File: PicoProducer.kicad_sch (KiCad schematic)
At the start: 37 parts, among them SW1 cherry_mx, SW10 cherry_mx, SW11 cherry_mx, SW12 cherry_mx, SW2 cherry_mx, SW3 cherry_mx, SW4 cherry_mx, SW5 cherry_mx, SW6 cherry_mx, SW7 cherry_mx, SW8 cherry_mx, SW9 cherry_mx, U1 RPI_PICO-SMD

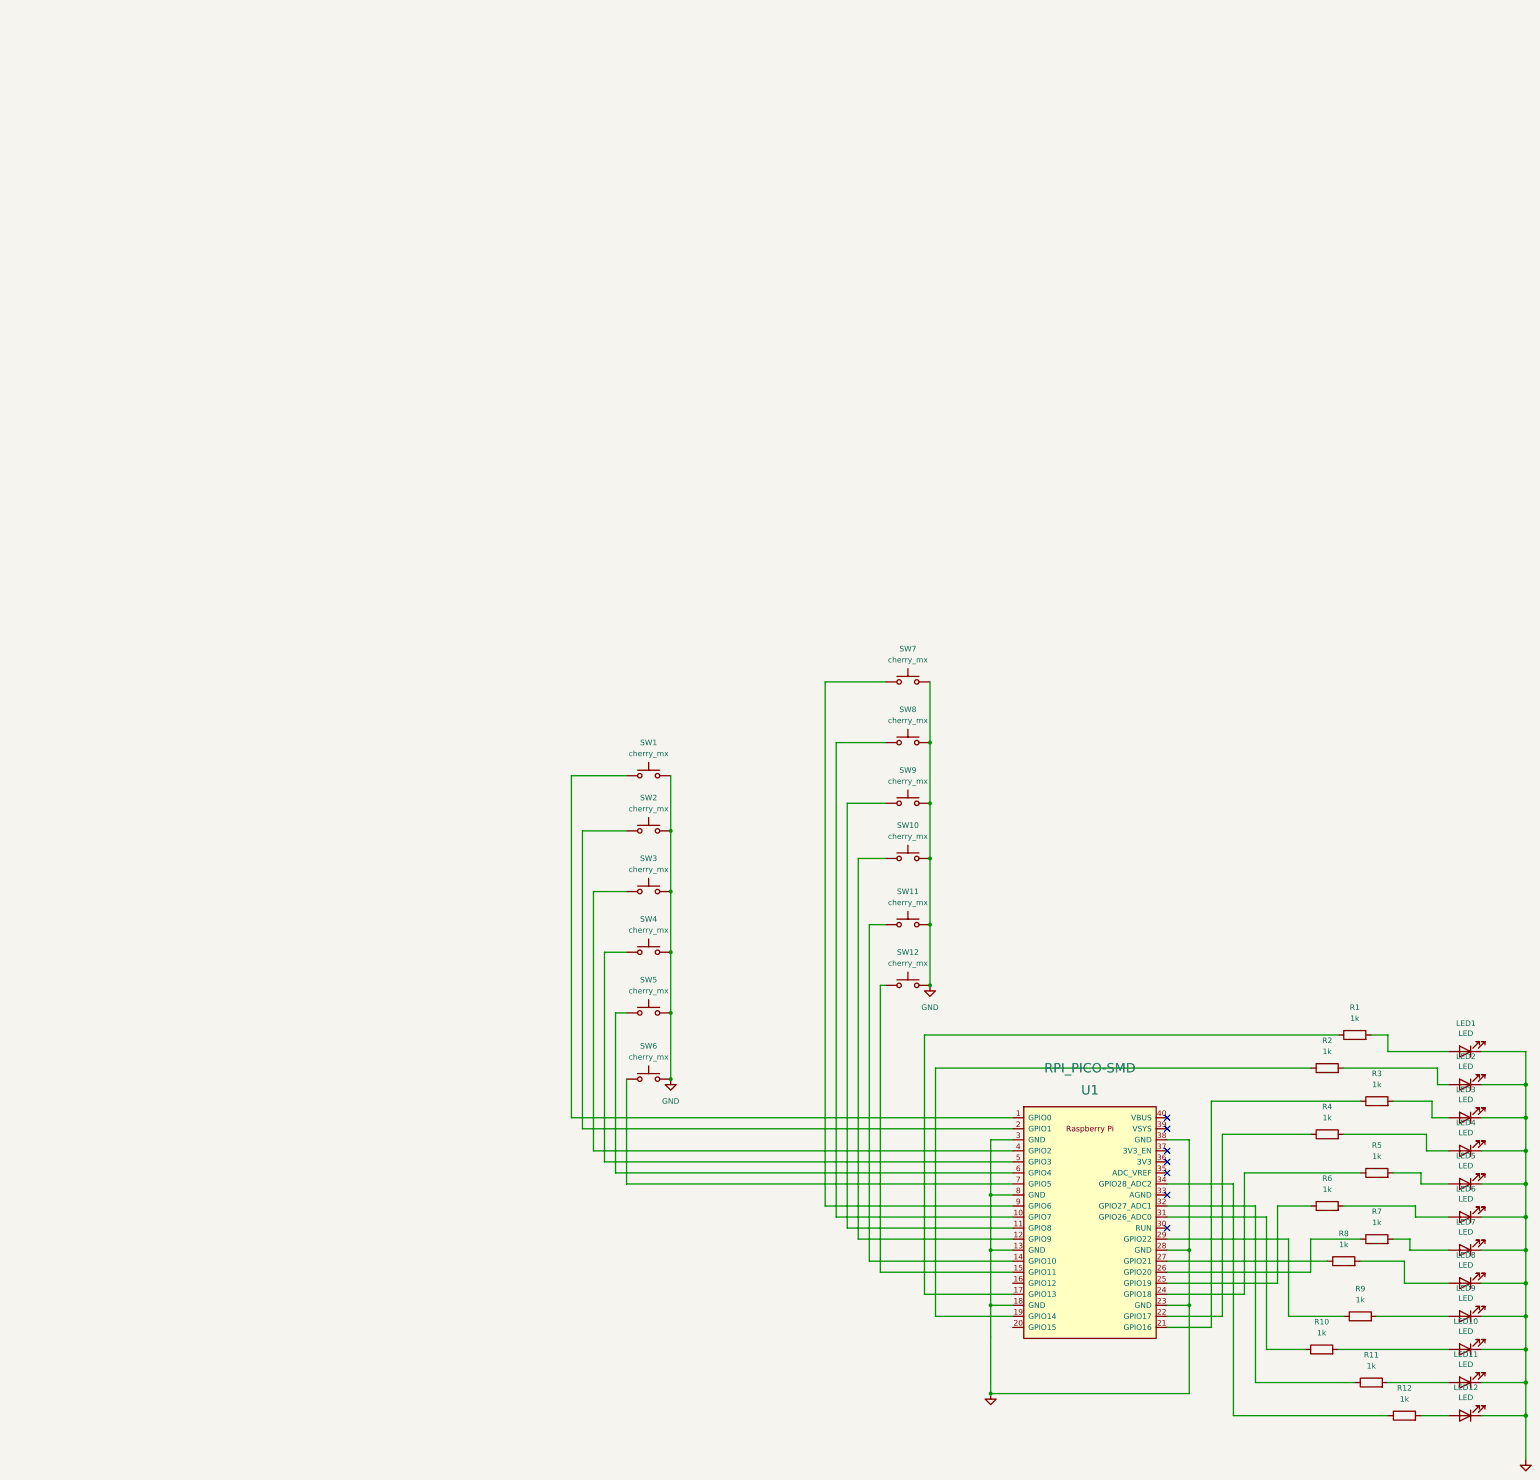
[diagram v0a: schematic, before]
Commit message: 0.2
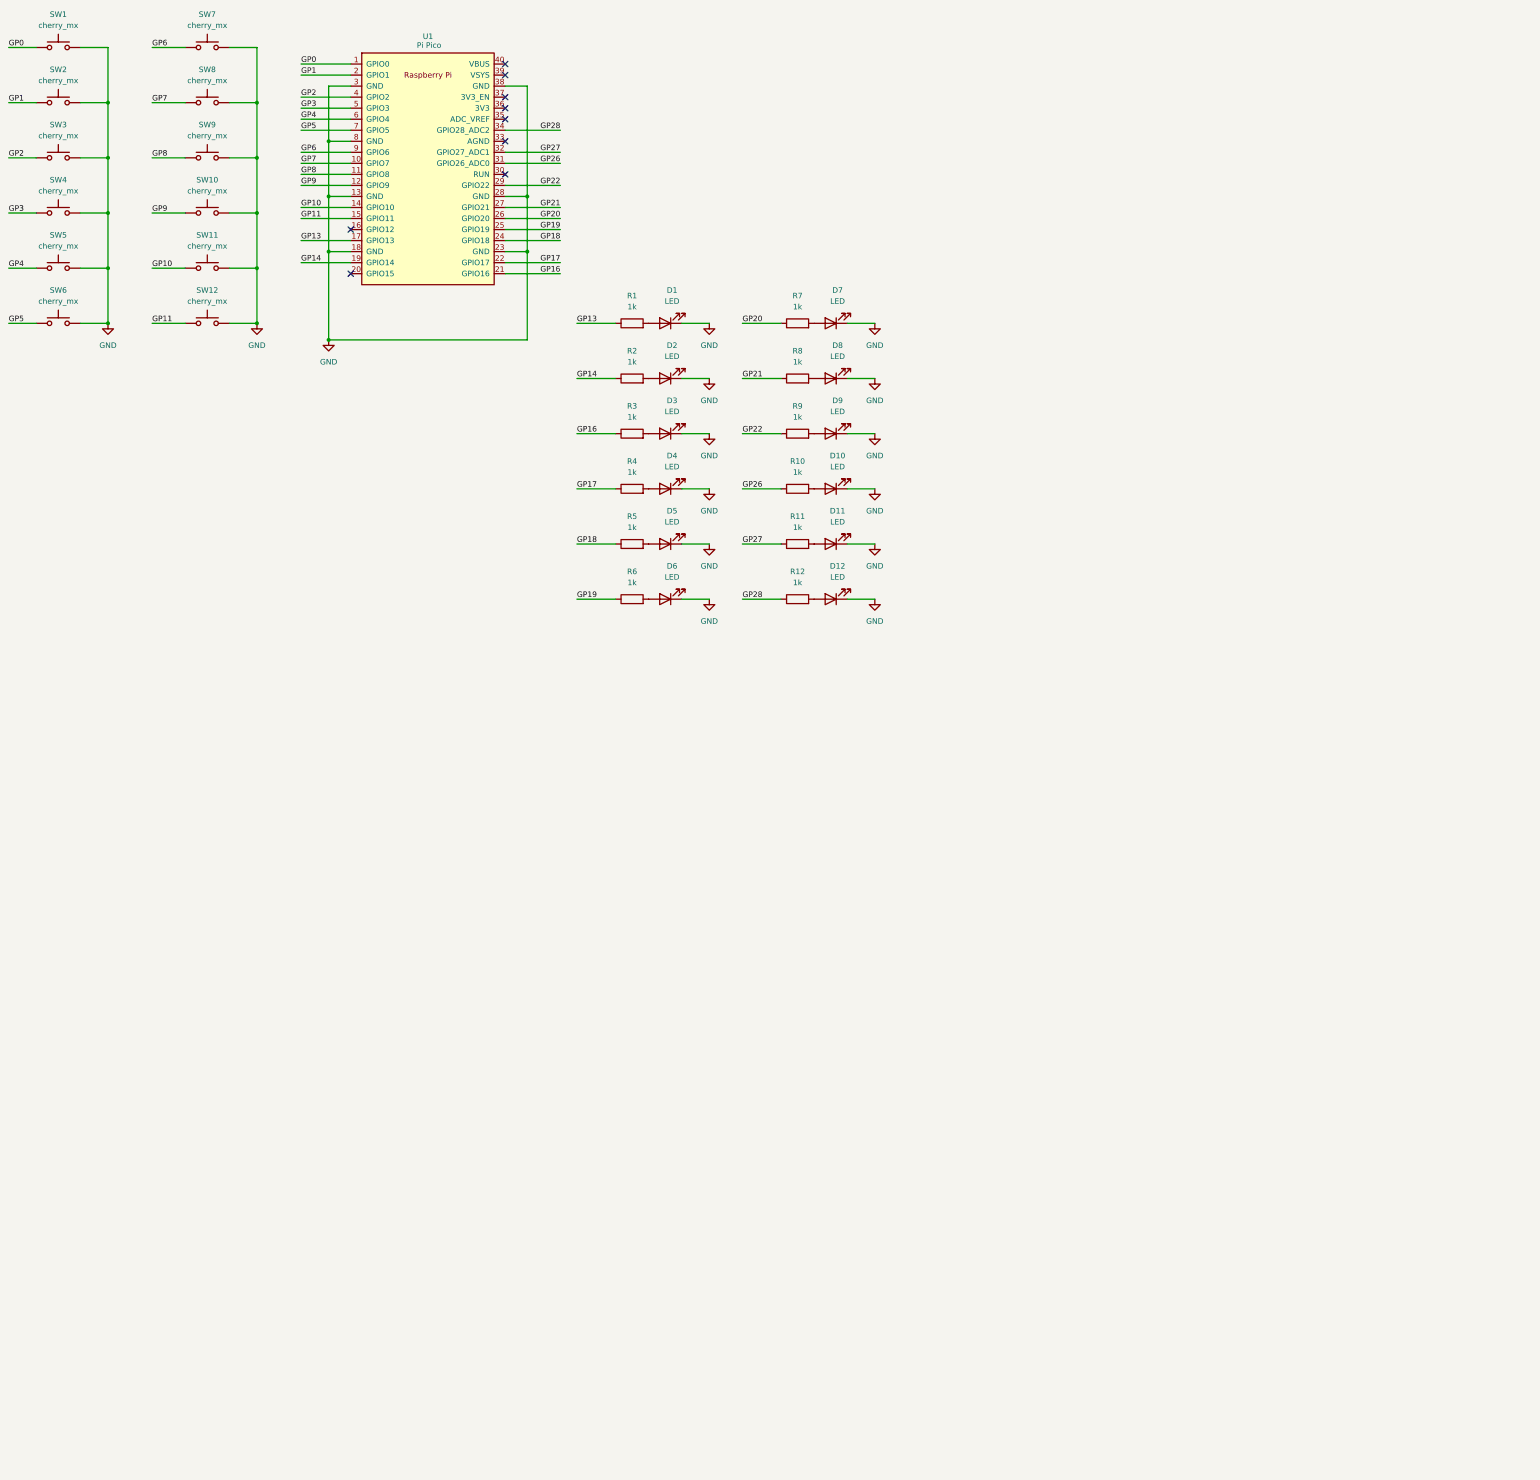
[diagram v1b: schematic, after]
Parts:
- removed LED1, LED10, LED11, LED12, LED2, LED3, LED4, LED5, LED6, LED7, LED8, LED9: LED, LED_THT:LED_D3.0mm, symbol PicoProducer-rescue:LED-Device
- added D1, D10, D11, D12, D2, D3, D4, D5, D6, D7, D8, D9: LED, LED_SMD:LED_0805_2012Metric_Pad1.15x1.40mm_HandSolder, symbol Device:LED
- R1, R10, R11, R12, R2, R3, R4, R5, R6, R7, R8, R9: footprint Resistor_THT:R_Axial_DIN0207_L6.3mm_D2.5mm_P7.62mm_Horizontal -> Resistor_SMD:R_0805_2012Metric_Pad1.20x1.40mm_HandSolder
- U1: value RPI_PICO-SMD -> Pi Pico; footprint Raspberry Pi:RPi_Pico_SMD_TH -> pi-pico:YD-RP2040
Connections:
- net GND: now also D1.1 (K), D10.1 (K), D11.1 (K), D12.1 (K), D2.1 (K), D3.1 (K), D4.1 (K), D5.1 (K), D6.1 (K), D7.1 (K), D8.1 (K), D9.1 (K)
- net at R1.2: now also D1.2 (A)
- net GP0: now reaches SW1.1, U1.1 (GPIO0)
- net GP7: now reaches SW8.1, U1.10 (GPIO7)
- net GP8: now reaches SW9.1, U1.11 (GPIO8)
- net GP9: now reaches SW10.1, U1.12 (GPIO9)
- net GP10: now reaches SW11.1, U1.14 (GPIO10)
- net GP11: now reaches SW12.1, U1.15 (GPIO11)
- net GP13: now reaches R1.1, U1.17 (GPIO13)
- net GP14: now reaches R2.1, U1.19 (GPIO14)
- net GP1: now reaches SW2.1, U1.2 (GPIO1)
- net GP16: now reaches R3.1, U1.21 (GPIO16)
- net GP17: now reaches R4.1, U1.22 (GPIO17)
- net GP18: now reaches R5.1, U1.24 (GPIO18)
- net GP19: now reaches R6.1, U1.25 (GPIO19)
- net GP20: now reaches R7.1, U1.26 (GPIO20)
- net GP21: now reaches R8.1, U1.27 (GPIO21)
- net GP22: now reaches R9.1, U1.29 (GPIO22)
- net GP26: now reaches R10.1, U1.31 (GPIO26_ADC0)
- net GP27: now reaches R11.1, U1.32 (GPIO27_ADC1)
- net GP28: now reaches R12.1, U1.34 (GPIO28_ADC2)
- net GP2: now reaches SW3.1, U1.4 (GPIO2)
- net GP3: now reaches SW4.1, U1.5 (GPIO3)
- net GP4: now reaches SW5.1, U1.6 (GPIO4)
- net GP5: now reaches SW6.1, U1.7 (GPIO5)
- net GP6: now reaches SW7.1, U1.9 (GPIO6)
- net at R2.2: now also D2.2 (A)
- net at R5.2: now also D5.2 (A)
- net at R3.2: now also D3.2 (A)
- net at R10.2: now also D10.2 (A)
- net at R9.2: now also D9.2 (A)
- net at R4.2: now also D4.2 (A)
- net at R11.2: now also D11.2 (A)
- net at R12.2: now also D12.2 (A)
- net at R7.2: now also D7.2 (A)
- net at R8.2: now also D8.2 (A)
- net at R6.2: now also D6.2 (A)
- no-connect marks 7 -> 9
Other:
- moved on the sheet: SW1, SW10, SW11, SW12, SW2, SW3, SW4, SW5, SW6, SW7, SW8, SW9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
